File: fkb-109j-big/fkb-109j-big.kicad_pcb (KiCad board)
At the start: 2 copper layers, 429.1 x 119.3 mm, 281 parts, among them J1 Conn_02x07_Counter_Clockwise, J10 Conn_01x04, J2 Conn_02x07_Counter_Clockwise, J3 Conn_01x01_Pin, J4 Conn_01x01_Pin, J5 Conn_01x05, J6 Conn_01x05, J7 Conn_01x05, J8 Conn_01x03, J9 Conn_01x03

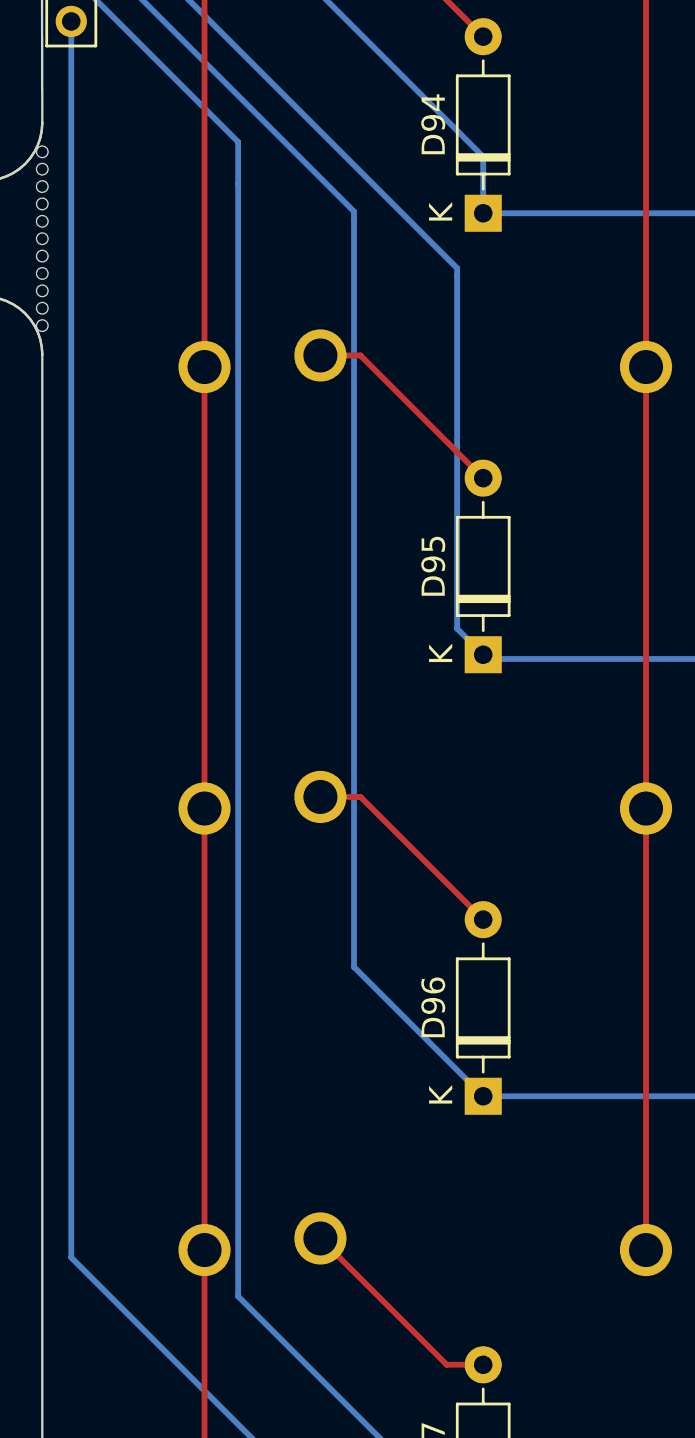
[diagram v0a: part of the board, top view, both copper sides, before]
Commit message: add teardrops.
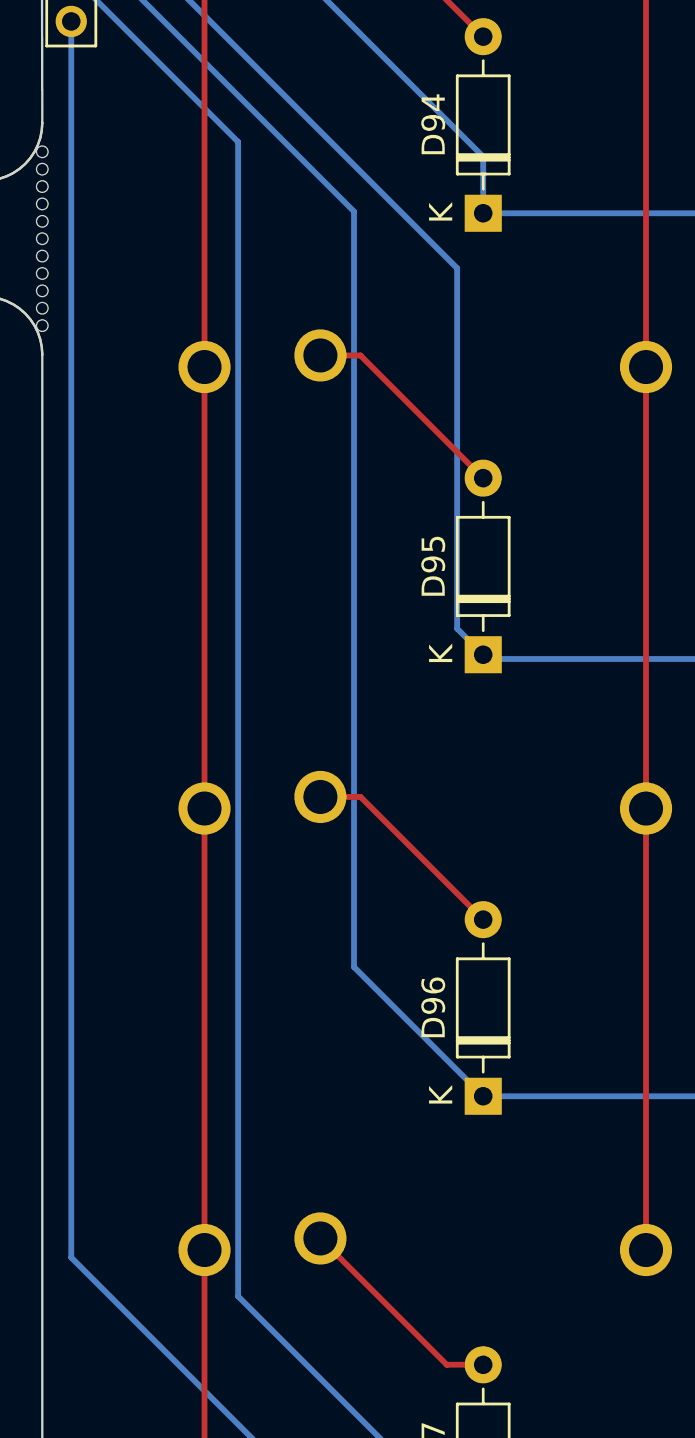
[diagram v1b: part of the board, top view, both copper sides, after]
